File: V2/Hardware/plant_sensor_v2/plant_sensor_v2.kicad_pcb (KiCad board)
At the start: 4 copper layers, 24.7 x 24.7 mm, 43 parts, among them IC1 ICM-20948, IC3 MLPF-NRG-01D3, J1 TC2030_SWD-MCP-NL, U2 TPS22960RSER, U3 TPS62840DLCR, U4 STM32WB09KEVx, Y1 520-.327-6-1210-TR (32.768kHz), Y2 NX1612SA-32.000MHZ-CHP-CIS-3

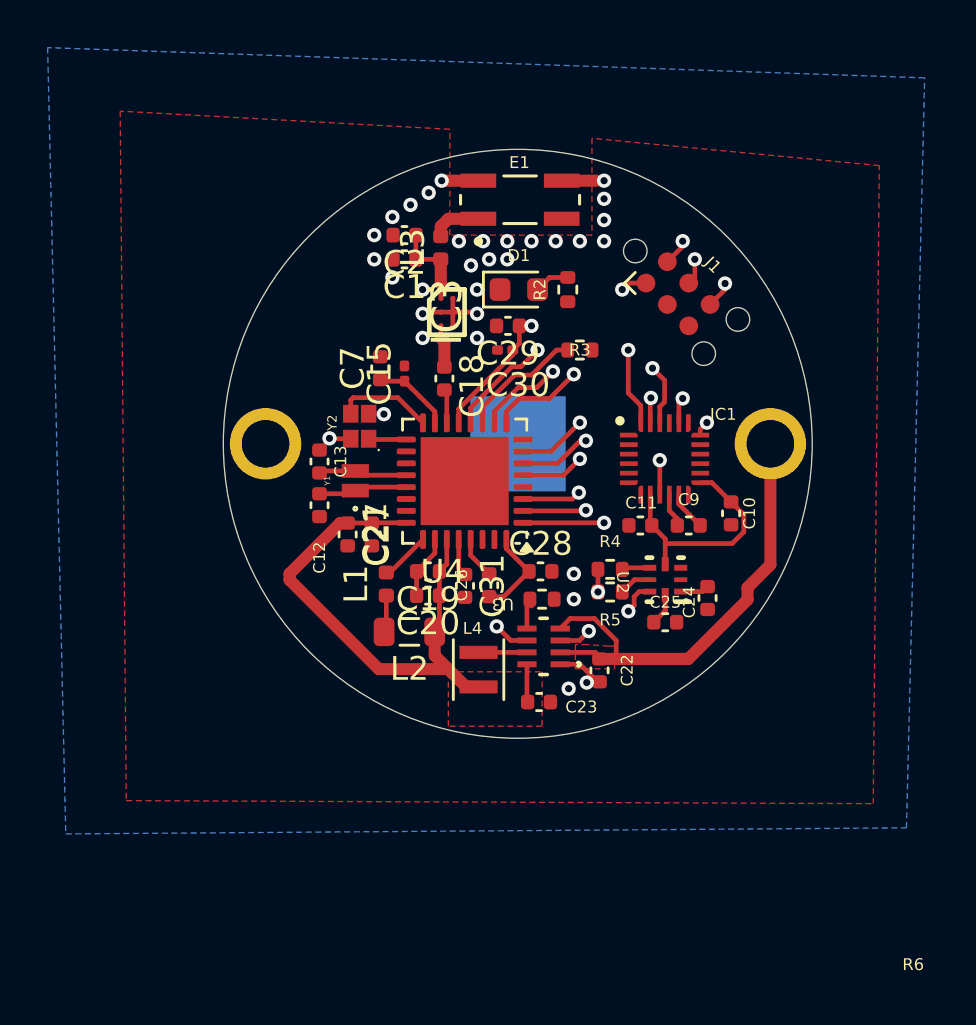
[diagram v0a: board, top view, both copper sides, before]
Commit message: Hardware design, almost finished
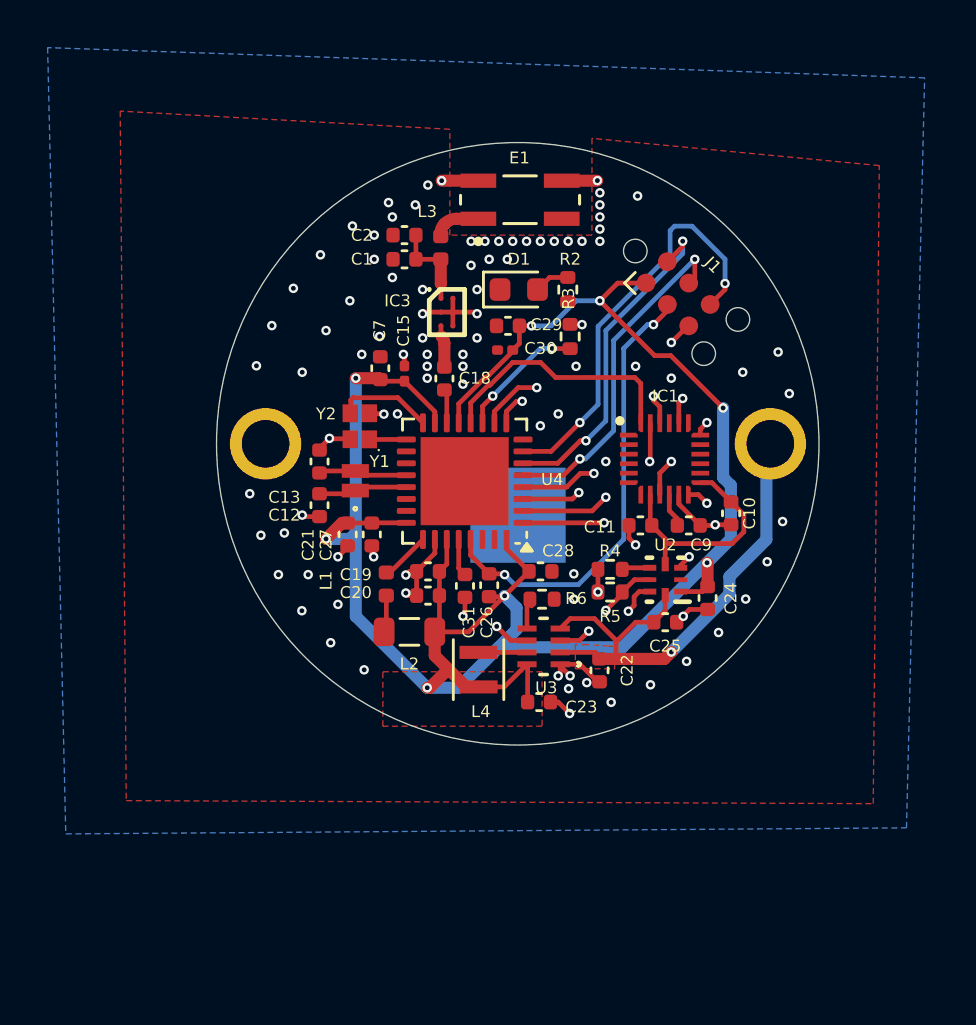
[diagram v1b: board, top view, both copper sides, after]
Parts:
- moved R3 0.70 mm to (105.0, 67.2), turned to 90 degrees
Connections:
- B1 pad 2: +BATT -> unconnected-(B1-Pad2)
- U4 pad 2: /BATT_EN -> /IMU_INT
- U4 pad 4: unconnected-(U4-PB0-Pad4) -> /BATT_EN
- U4 pad 8: /IMU_INT -> unconnected-(U4-PA0-Pad8)
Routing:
- net +1V8: track 42.5 -> 87.9 mm, vias 2 -> 8
- net /~{RESET}: track 1.76 -> 19.2 mm, vias 0 -> 2
- net GND: track 20.6 -> 35.0 mm, vias 36 -> 102
- net /IMU_INT: track 0.00 -> 8.99 mm, vias 0 -> 2
- net /SCLK: track 10.6 -> 8.39 mm
- net /BATT_EN: track 9.09 -> 11.1 mm
- net /MISO: track 12.6 -> 10.6 mm
- net /~{SS}: track 10.7 -> 8.97 mm
- net +BATT: track 20.9 -> 22.2 mm, vias 0 -> 1
- net /MOSI: track 12.0 -> 10.7 mm, vias 2 -> 0
- net Net-(U4-PA10): track 5.23 -> 5.38 mm, vias 0 -> 2
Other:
- board size 24.7 x 24.7 mm -> 25.3 x 25.3 mm
